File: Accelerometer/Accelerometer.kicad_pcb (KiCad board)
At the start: 2 copper layers, 50 x 31 mm, 6 parts, among them J1 M80-8770405, U1 KX134-1211

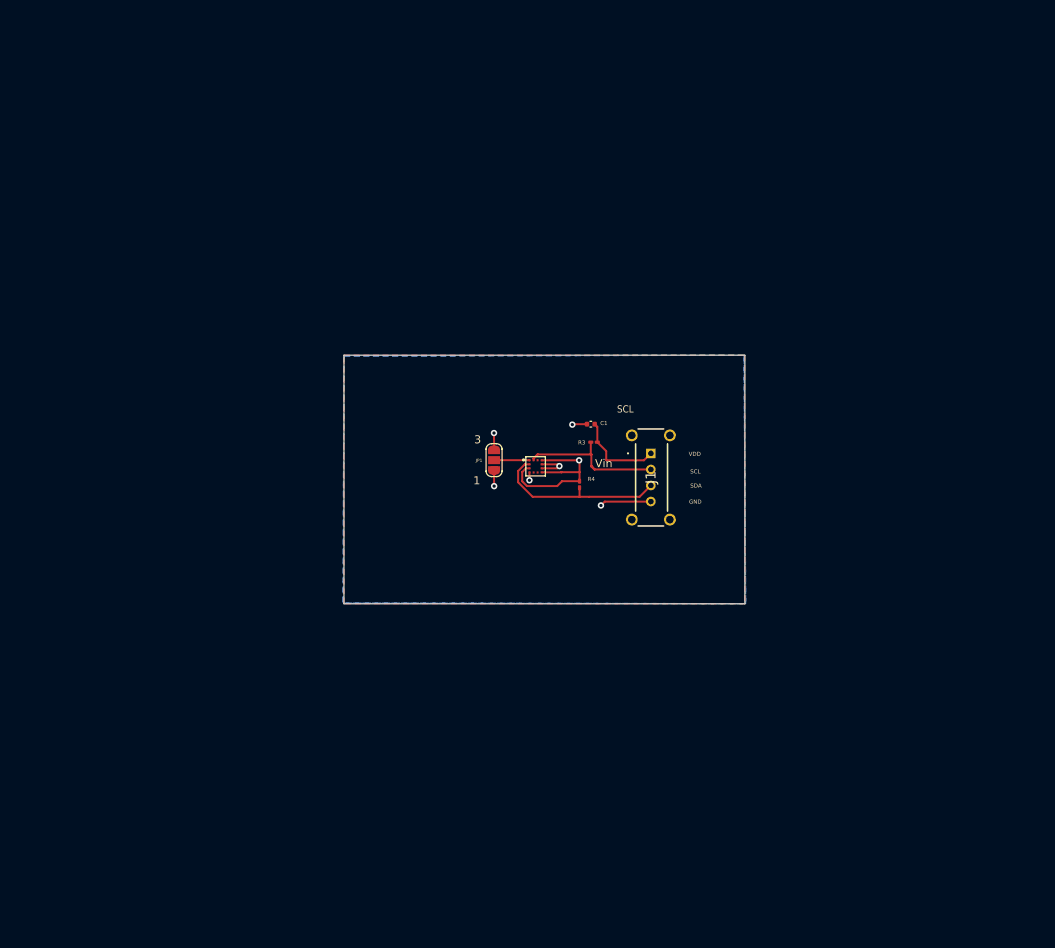
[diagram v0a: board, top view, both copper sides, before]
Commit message: LC24 PCBs
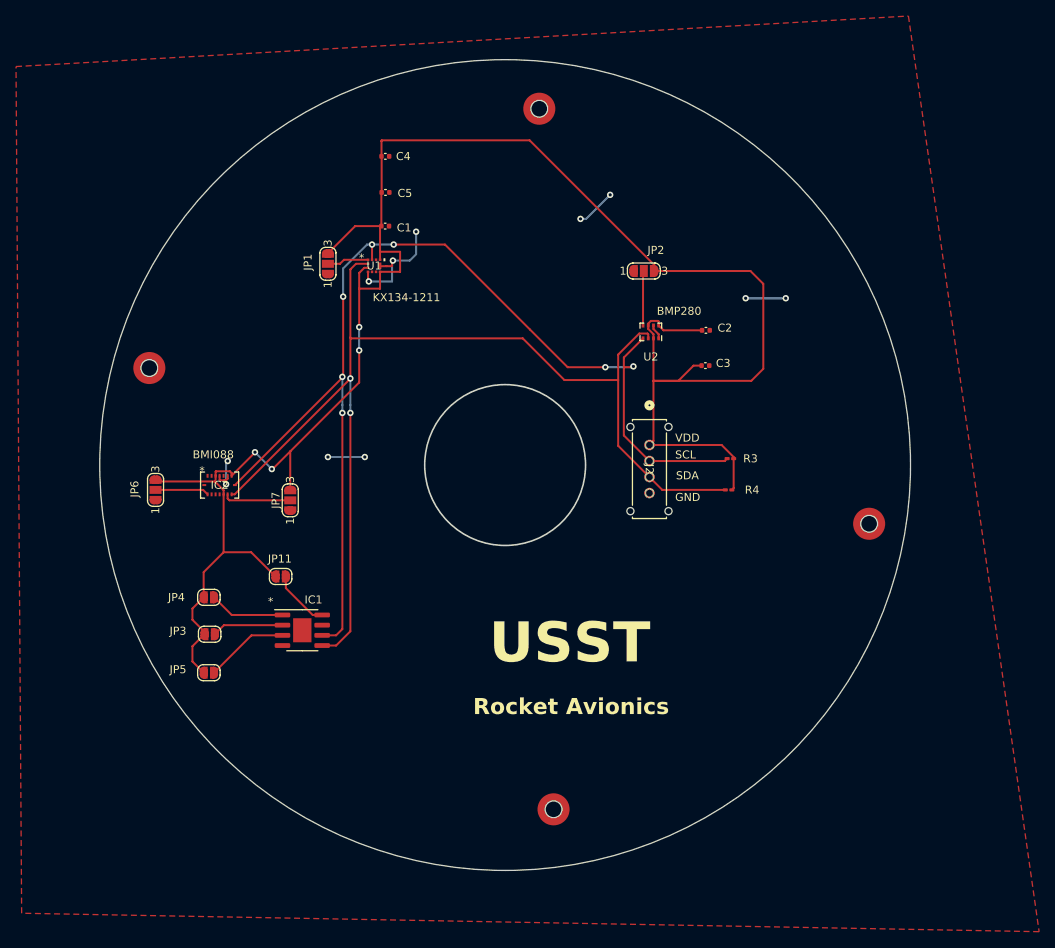
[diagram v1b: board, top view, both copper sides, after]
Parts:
- removed J1: M80-8770405, KiCad:M808770405
- added C2: 100nF, Capacitor_SMD:C_0402_1005Metric, F.Cu at (157.9, 73.3)
- added C3: 100nF, Capacitor_SMD:C_0402_1005Metric, F.Cu at (157.9, 77.7)
- added C4: 100n, Capacitor_SMD:C_0402_1005Metric, F.Cu at (118.0, 51.6)
- added C5: 100n, Capacitor_SMD:C_0402_1005Metric, F.Cu at (118.0, 56.1)
- added H1: MountingHole_Pad, Mounting_Wuerth:Mounting_Wuerth_WA-SMSI-M1.6_H1mm_9774010633, F.Cu at (137.2, 45.7)
- added H2: MountingHole_Pad, Mounting_Wuerth:Mounting_Wuerth_WA-SMSI-M1.6_H1mm_9774010633, F.Cu at (138.9, 133.0)
- added H3: MountingHole_Pad, Mounting_Wuerth:Mounting_Wuerth_WA-SMSI-M1.6_H1mm_9774010633, F.Cu at (88.5, 78.0)
- added H4: MountingHole_Pad, Mounting_Wuerth:Mounting_Wuerth_WA-SMSI-M1.6_H1mm_9774010633, F.Cu at (178.3, 97.4)
- added IC1: FRAM, Package_SO:SOIC-8-1EP_3.9x4.9mm_P1.27mm_EP2.29x3mm, F.Cu at (107.6, 110.7)
- added IC2: BMI088, BMI088:QFN_BMI085_BOS, F.Cu at (97.3, 92.6)
- added J2: M80-8770422, Harwin-M80-8770422:CONN_M80-87704_HRW, F.Cu at (150.9, 87.6)
- added JP11: SolderJumper_2_Open, Jumper:SolderJumper-2_P1.3mm_Open_RoundedPad1.0x1.5mm, F.Cu at (104.9, 104.0)
- added JP2: SolderJumper_3_Open, Jumper:SolderJumper-3_P1.3mm_Open_RoundedPad1.0x1.5mm_NumberLabels, F.Cu at (150.2, 65.9)
- added JP3: SolderJumper_2_Open, Jumper:SolderJumper-2_P1.3mm_Open_RoundedPad1.0x1.5mm, F.Cu at (96.0, 111.2)
- added JP4: SolderJumper_2_Open, Jumper:SolderJumper-2_P1.3mm_Open_RoundedPad1.0x1.5mm, F.Cu at (96.0, 106.6)
- added JP5: SolderJumper_2_Open, Jumper:SolderJumper-2_P1.3mm_Open_RoundedPad1.0x1.5mm, F.Cu at (96.0, 116.0)
- added JP6: SolderJumper_3_Open, Jumper:SolderJumper-3_P1.3mm_Open_RoundedPad1.0x1.5mm_NumberLabels, F.Cu at (89.3, 93.2)
- added JP7: SolderJumper_3_Open, Jumper:SolderJumper-3_P1.3mm_Open_RoundedPad1.0x1.5mm_NumberLabels, F.Cu at (106.1, 94.5)
- added U2: BMP280, Package_LGA:Bosch_LGA-8_2x2.5mm_P0.65mm_ClockwisePinNumbering, F.Cu at (151.1, 73.5)
- U1: footprint XDCR_KX003-1077:XDCR_KX003-1077 -> KX134:LGA12_2X2X0P9_ROM
- moved C1 35.6 mm to (117.9, 60.3), turned to 0 degrees
- moved U1 32.1 mm to (116.6, 65.3)
- moved JP1 32.1 mm to (110.8, 65.0)
- moved R4 18.6 mm to (160.8, 93.2), turned to 180 degrees
- moved R3 17.1 mm to (161.0, 89.3)
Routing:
- net +3.3V: track 35.1 -> 250.3 mm, vias 2 -> 4
- net /SCL: track 20.1 -> 141.5 mm, vias 0 -> 7
- net /SDA: track 22.2 -> 140.7 mm, vias 0 -> 2
- net GND: track 15.8 -> 37.7 mm, vias 5 -> 11
- net Net-(IC1-A2): track 0.00 -> 10.5 mm
- net Net-(IC1-A0): track 0.00 -> 9.44 mm
- net Net-(IC1-A1): track 0.00 -> 8.90 mm
- net Net-(IC2-SDO2): track 0.00 -> 8.42 mm
- net Net-(IC1-VDD): track 0.00 -> 7.37 mm
- net Net-(JP2-C): track 0.00 -> 6.84 mm
- net Net-(IC2-SDO1): track 0.00 -> 6.72 mm
- net Net-(JP1-C): track 4.43 -> 5.21 mm
- removed copper zone on B.Cu, net +3.3V
- removed copper zone on B.Cu, net GND
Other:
- board size 50 x 31 mm -> 101.1 x 101.1 mm
- board text added: "Rocket Avionics"
- board text added: "USST"
- board text removed: "Vin"
